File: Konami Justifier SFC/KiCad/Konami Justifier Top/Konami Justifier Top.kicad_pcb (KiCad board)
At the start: 4 copper layers, 15.2 x 50 mm, 10 parts, among them J1 RJ12, U1 IS485

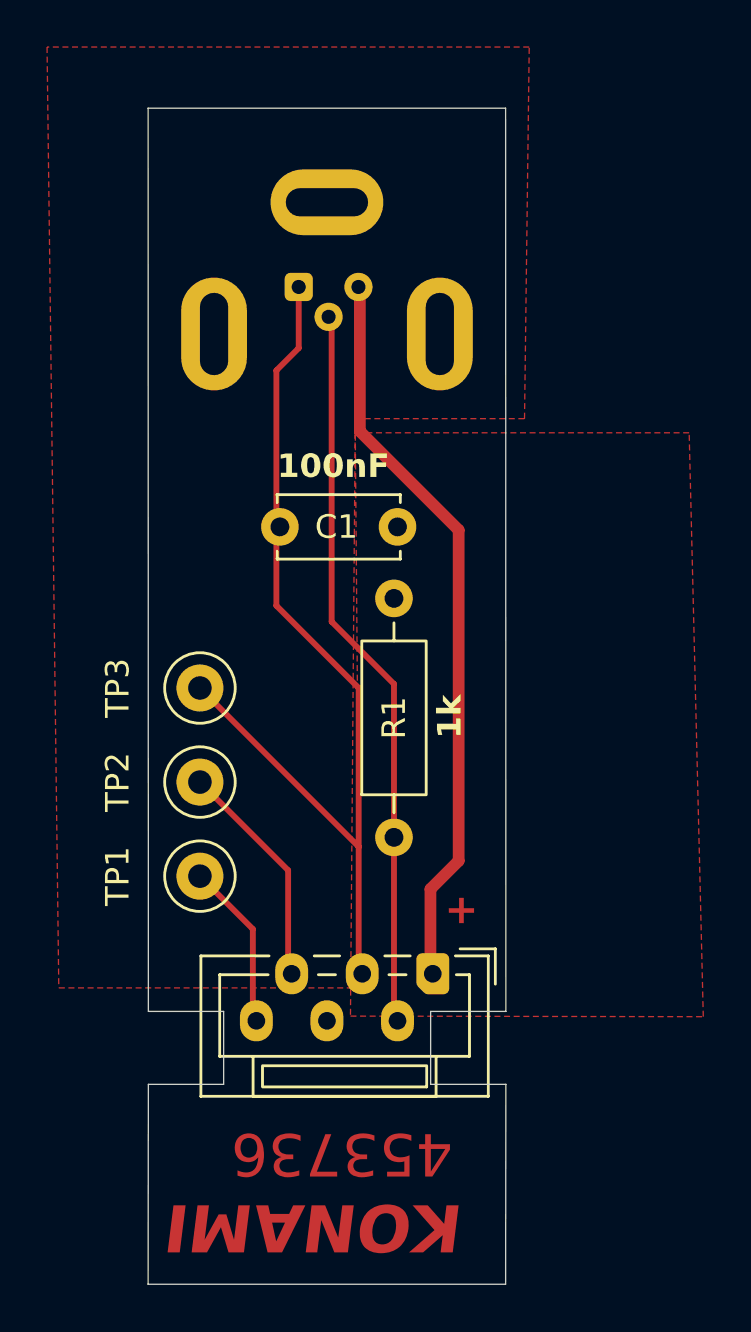
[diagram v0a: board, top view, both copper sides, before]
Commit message: Add files via upload
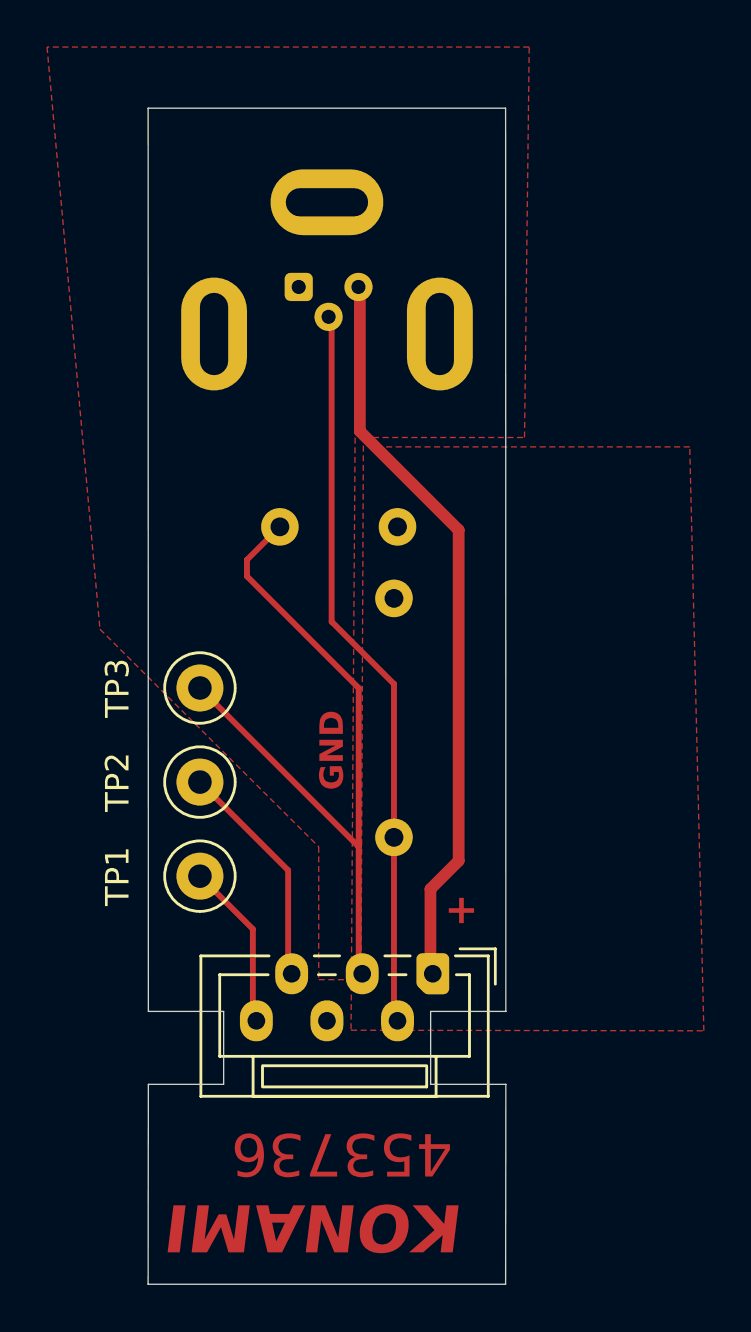
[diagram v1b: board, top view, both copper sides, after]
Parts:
- C1, R1: moved to B.Cu
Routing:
- net GND: track 40.4 -> 30.9 mm
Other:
- board text added: "GND"
